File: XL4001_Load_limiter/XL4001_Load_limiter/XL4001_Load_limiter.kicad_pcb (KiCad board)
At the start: 2 copper layers, 49 x 51 mm, 34 parts, among them J1 5.08-2P-90, J2 5.08-2P-90, J3 Conn_01x02_Socket, Q1 PMOS, Q2 2N7002K, U1 XL4001

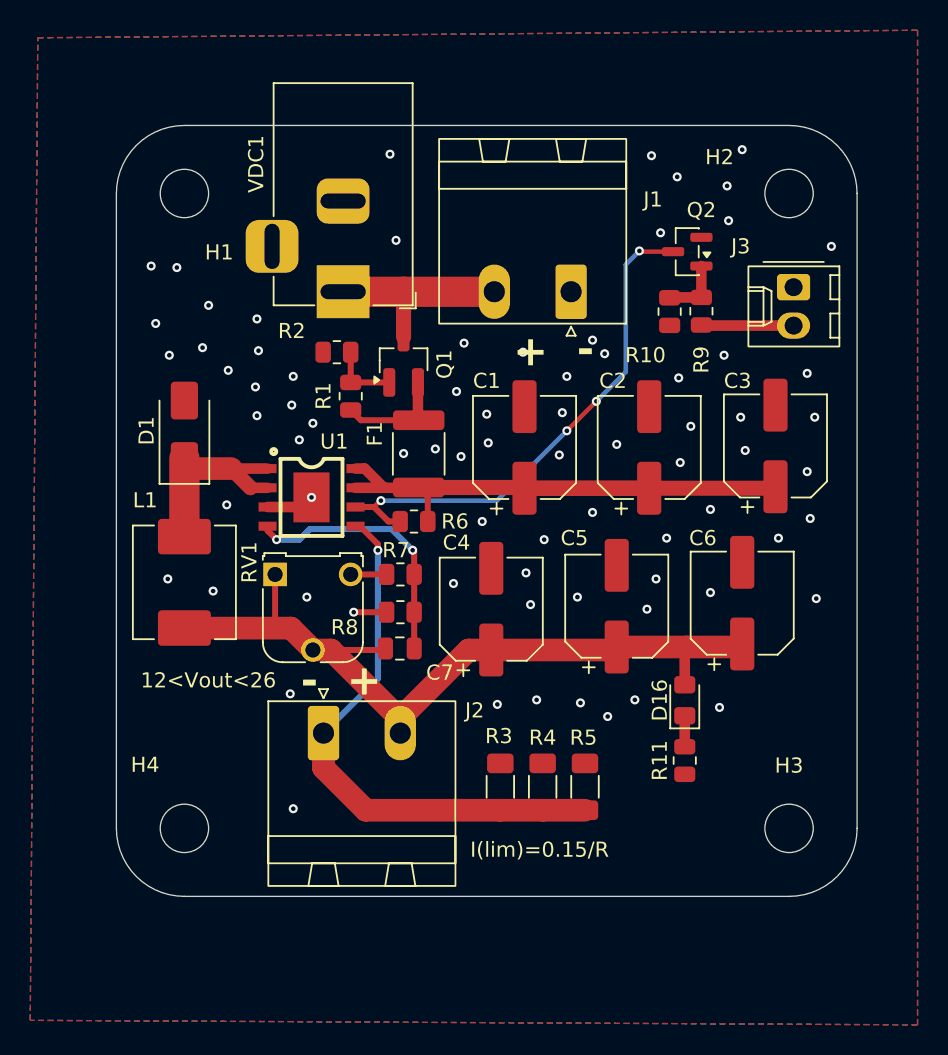
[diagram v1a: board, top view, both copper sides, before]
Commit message: Sincronização de arquivos
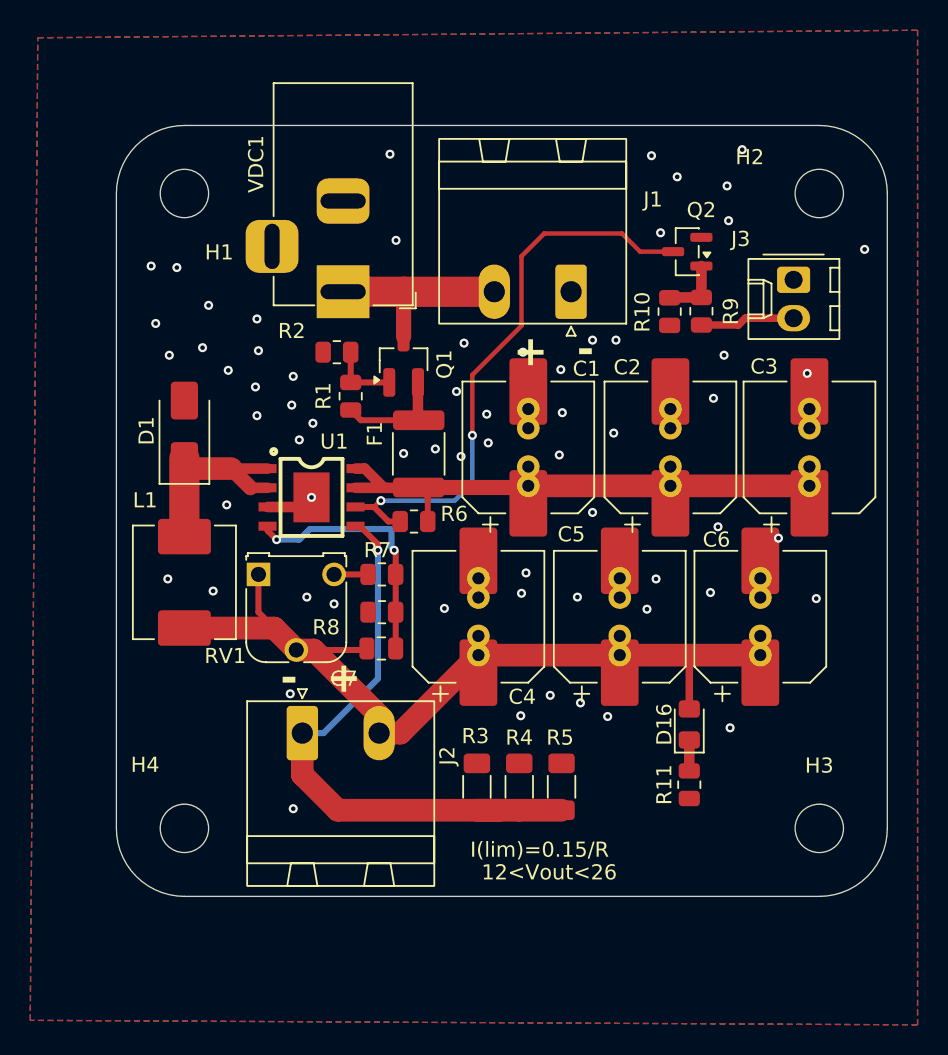
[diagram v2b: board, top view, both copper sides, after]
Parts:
- C1, C2, C3, C4, C5, C6: footprint Capacitor_SMD:CP_Elec_6.3x7.7 -> Aleoexpress:Cap_polymer
- moved C3 2.25 mm to (163.7, 77.6)
- moved H2 2.00 mm to (164.3, 60.8)
- moved H3 2.00 mm to (164.3, 102.8)
- moved D16 1.63 mm to (155.7, 95.9)
- moved R11 1.63 mm to (155.7, 99.9)
- moved R4 1.55 mm to (144.4, 100.0)
- moved R5 1.55 mm to (147.2, 100.0)
- moved R3 1.55 mm to (141.7, 100.0)
- moved C6 1.50 mm to (160.4, 88.8)
- moved J2 1.40 mm to (130.1, 96.5)
- moved C2 1.40 mm to (154.4, 77.6)
- moved C7 1.23 mm to (135.3, 90.9)
- moved R7 1.23 mm to (135.4, 86.0)
- moved R8 1.23 mm to (135.4, 88.5)
- moved RV1 1.10 mm to (127.2, 86.0)
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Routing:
- net VCC: track 41.0 -> 34.7 mm
- net EN_CH0: track 34.3 -> 38.0 mm, vias 4 -> 2
- net PCH0: track 55.5 -> 58.6 mm
- net NCH0: track 36.7 -> 39.8 mm
- net GND: track 5.35 -> 3.17 mm, vias 76 -> 65
- net FB_CH0: track 17.5 -> 17.0 mm
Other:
- board size 49 x 51 mm -> 51 x 51 mm
